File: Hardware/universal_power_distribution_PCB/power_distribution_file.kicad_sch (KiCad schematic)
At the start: 13 parts, among them J1 Screw_Terminal_01x02, U2 INA228

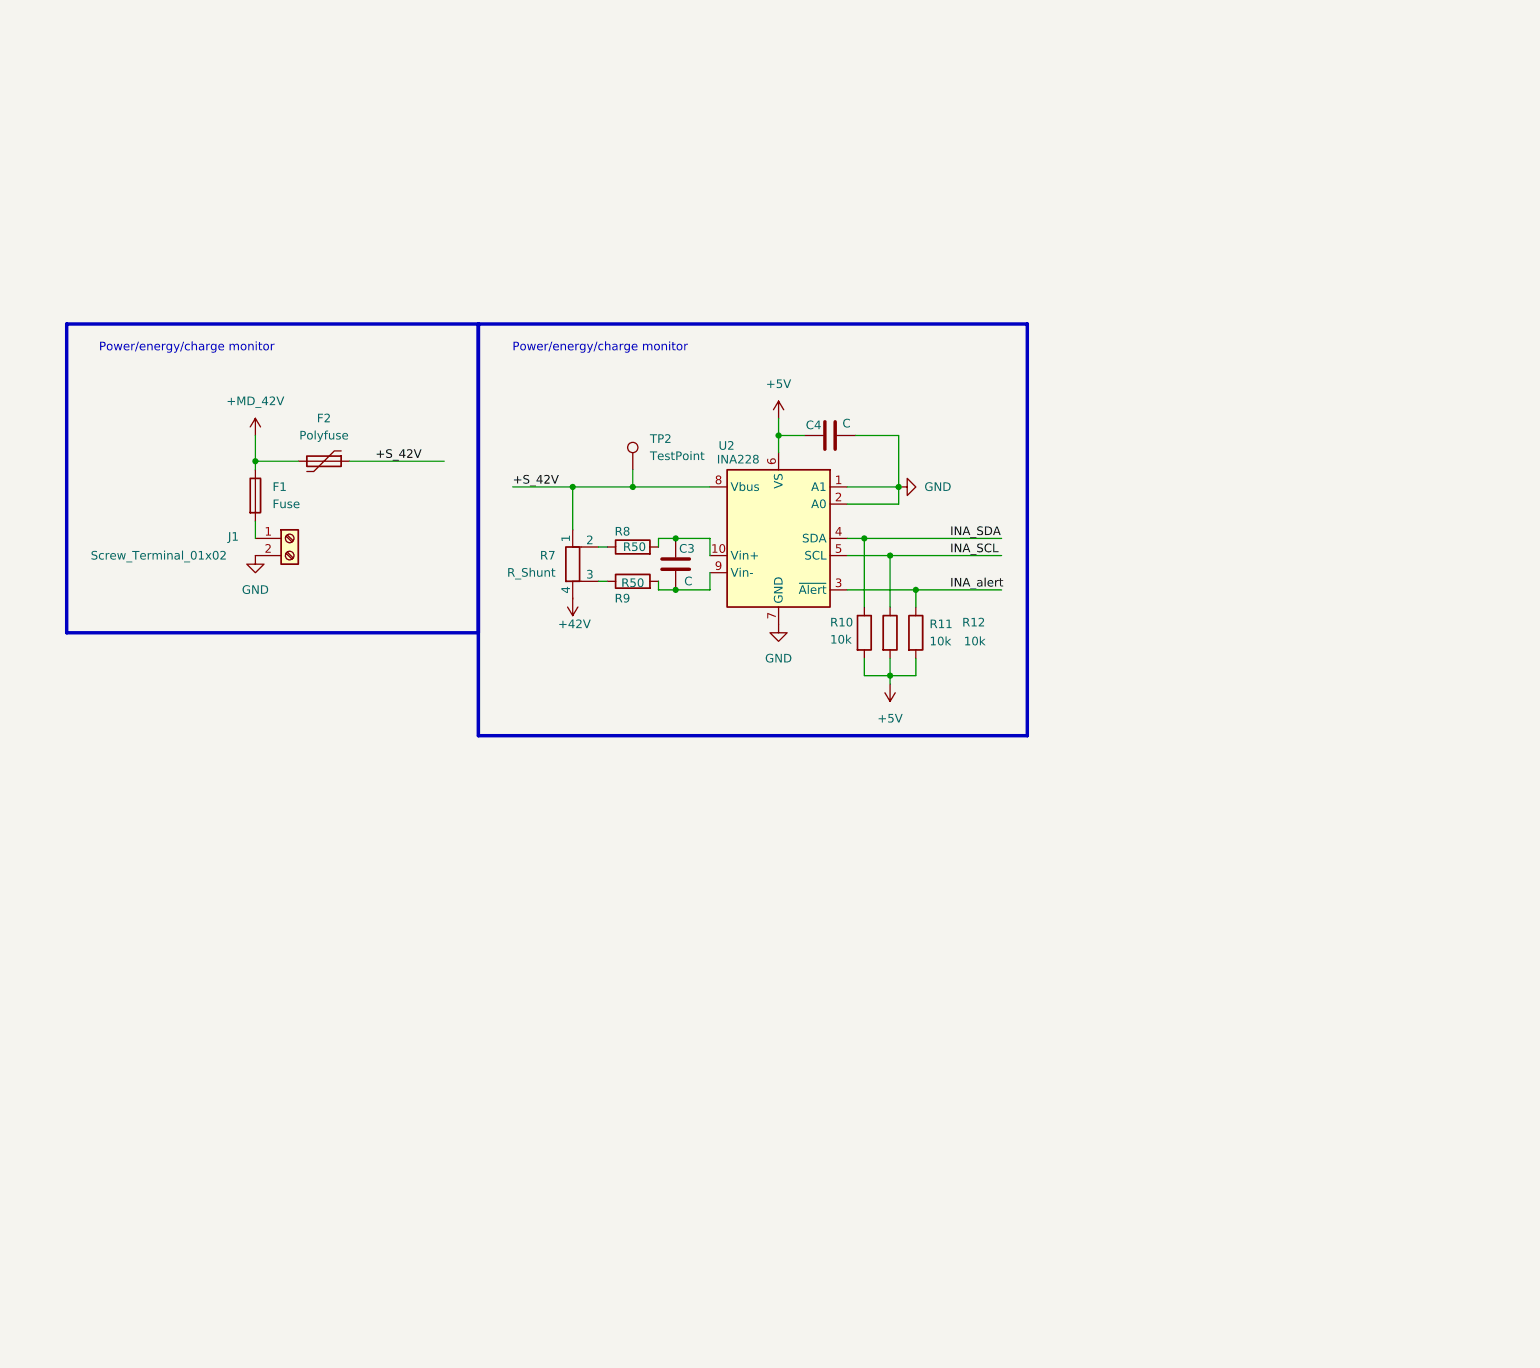
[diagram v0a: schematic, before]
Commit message: Updated universal PCB
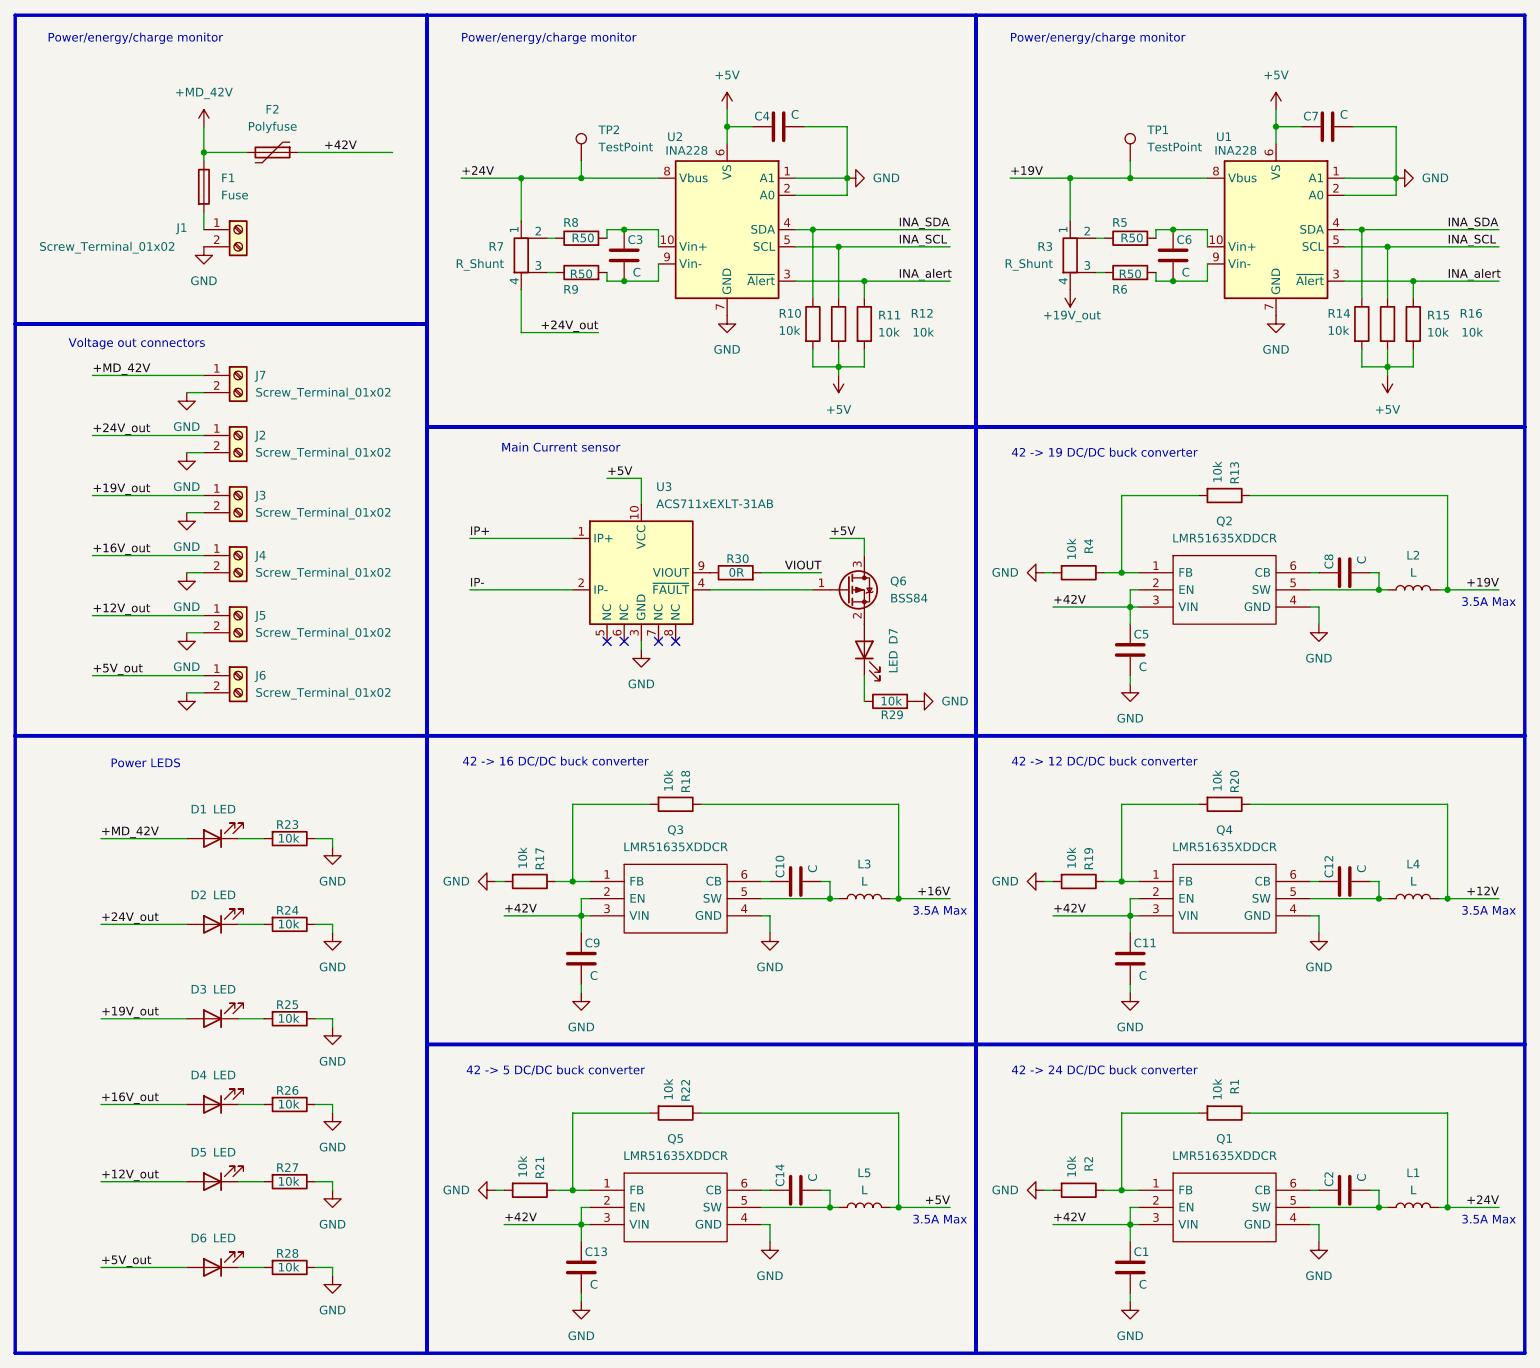
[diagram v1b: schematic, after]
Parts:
- added C1, C10, C11, C12, C13, C14, C2, C5, C6, C7, C8, C9: C, symbol Device:C
- added D1, D2, D3, D4, D5, D6, D7: LED, symbol Device:LED
- added J2, J3, J4, J5, J6, J7: Screw_Terminal_01x02, symbol Connector:Screw_Terminal_01x02
- added L1, L2, L3, L4, L5: L, symbol Device:L
- added Q1, Q2, Q3, Q4, Q5: LMR51635XDDCR, SOT95P280X110-6N, symbol LMR51635XDDCR:LMR51635XDDCR
- added Q6: BSS84, Package_TO_SOT_SMD:SOT-23, symbol Transistor_FET:BSS84
- added R1, R13, R14, R15, R16, R17, R18, R19, R2, R20, R21, R22, R23, R24, R25, R26, R27, R28, R29, R4: 10k, symbol Device:R
- added R3: R_Shunt, symbol Device:R_Shunt
- added R30: 0R, symbol Device:R
- added R5, R6: R50, symbol Device:R
- added TP1: TestPoint, symbol Connector:TestPoint
- added U1: INA228, Package_SO:VSSOP-10_3x3mm_P0.5mm, symbol Sensor_Energy:INA228
- added U3: ACS711xEXLT-31AB, Sensor_Current:Allegro_QFN-12-10-1EP_3x3mm_P0.5mm, symbol Sensor_Current:ACS711xEXLT-31AB
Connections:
- net +42V: now also F2.1, C1.1, C11.1, C13.1, C5.1, C9.1, Q1.2 (EN), Q1.3 (VIN), Q2.2 (EN), Q2.3 (VIN), Q3.2 (EN), Q3.3 (VIN), Q4.2 (EN), Q4.3 (VIN), Q5.2 (EN), Q5.3 (VIN); no longer R7.4
- net +5V: now also C7.1, L5.2, Q6.3 (D), R14.2, R15.2, R16.2, R22.1, U1.6 (VS), U3.10 (VCC)
- net +MD_42V: now also D1.2 (A), J7.1 (Pin_1)
- net GND: now also C1.2, C11.2, C13.2, C5.2, C7.2, C9.2, J2.2 (Pin_2), J3.2 (Pin_2), J4.2 (Pin_2), J5.2 (Pin_2), J6.2 (Pin_2), J7.2 (Pin_2), Q1.4 (GND), Q2.4 (GND), Q3.4 (GND), Q4.4 (GND), Q5.4 (GND), R17.2, R19.2, R2.2, R21.2, R23.1, R24.1, R25.1, R26.1, R27.1, R28.1, R29.2, R4.2, U1.1 (A1), U1.2 (A0), U1.7 (GND), U3.3 (GND)
- net INA_SCL: now also R15.1, U1.5 (SCL)
- net INA_SDA: now also R14.1, U1.4 (SDA)
- net INA_alert: now also R16.1, U1.3 (~{Alert})
- net +S_42V renamed +24V
- net +24V: now also L1.2, R1.1; no longer F2.1
- new net: R3.3, R6.1
- new net: C6.2, R6.2, U1.9 (Vin-)
- new net: Q4.1 (FB), R19.1, R20.2
- new net: D4.1 (K), R26.2
- new net: C12.2, L4.1, Q4.5 (SW)
- new net: C12.1, Q4.6 (CB)
- new net: C6.1, R5.2, U1.10 (Vin+)
- new net: Q2.1 (FB), R13.2, R4.1
- new net: C2.1, Q1.6 (CB)
- new net: C2.2, L1.1, Q1.5 (SW)
- new net: R3.2, R5.1
- new net: C8.2, L2.1, Q2.5 (SW)
- new net: C10.2, L3.1, Q3.5 (SW)
- new net: Q6.1 (G), U3.4 (~{FAULT})
- new net: R30.1, U3.9 (VIOUT)
- new net: D3.1 (K), R25.2
- new net: D1.1 (K), R23.2
- new net: D5.1 (K), R27.2
- new net: D2.1 (K), R24.2
- new net: C8.1, Q2.6 (CB)
- new net: D7.1 (K), R29.1
- new net: C14.1, Q5.6 (CB)
- new net: C14.2, L5.1, Q5.5 (SW)
- new net: D7.2 (A), Q6.2 (S)
- new net: Q3.1 (FB), R17.1, R18.2
- new net: Q5.1 (FB), R21.1, R22.2
- new net: C10.1, Q3.6 (CB)
- new net: D6.1 (K), R28.2
- new net: Q1.1 (FB), R1.2, R2.1
- new net +12V: L4.2, R20.1
- new net +12V_out: D5.2 (A), J5.1 (Pin_1)
- new net +16V: L3.2, R18.1
- new net +16V_out: D4.2 (A), J4.1 (Pin_1)
- new net +19V: L2.2, R13.1, R3.1, TP1.1, U1.8 (Vbus)
- new net +19V_out: D3.2 (A), J3.1 (Pin_1), R3.4
- new net +24V_out: D2.2 (A), J2.1 (Pin_1), R7.4
- new net +5V_out: D6.2 (A), J6.1 (Pin_1)
- new net IP+: U3.1 (IP+)
- new net IP-: U3.2 (IP-)
- new net VIOUT: R30.2
- no-connect marks 0 -> 4
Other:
- note added: "3.5A Max"
- note added: "42 -> 12 DC/DC buck converter"
- note added: "42 -> 16 DC/DC buck converter"
- note added: "42 -> 19 DC/DC buck converter"
- note added: "42 -> 24 DC/DC buck converter"
- note added: "42 -> 5 DC/DC buck converter"
- note added: "Main Current sensor"
- note added: "Power LEDS"
- note added: "Voltage out connectors"
- company: (none) -> Lapin AMK
- title: (none) -> Power distribution pcb
- moved on the sheet: C3, C4, F1, F2, J1, R10, R11, R12, R7, R8, R9, TP2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
